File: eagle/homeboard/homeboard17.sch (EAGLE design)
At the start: 128 parts, among them IC1 XCF02S, IC2 25LC080SN, IC3 ATMEGA32U2-TQFP, Q5 BC848SMD, Q6 BC848SMD, Q7 BC848SMD, Q8 BC848SMD, T1 BSS138, T2 BC848, T3 BSS138, T4 BC848, U1 XC3S400TQ144, X1 SCART-CLIP, X6 MINI-USB_4P-85-32004-10X, X7 DC21MMX, X8 STEREOJACK

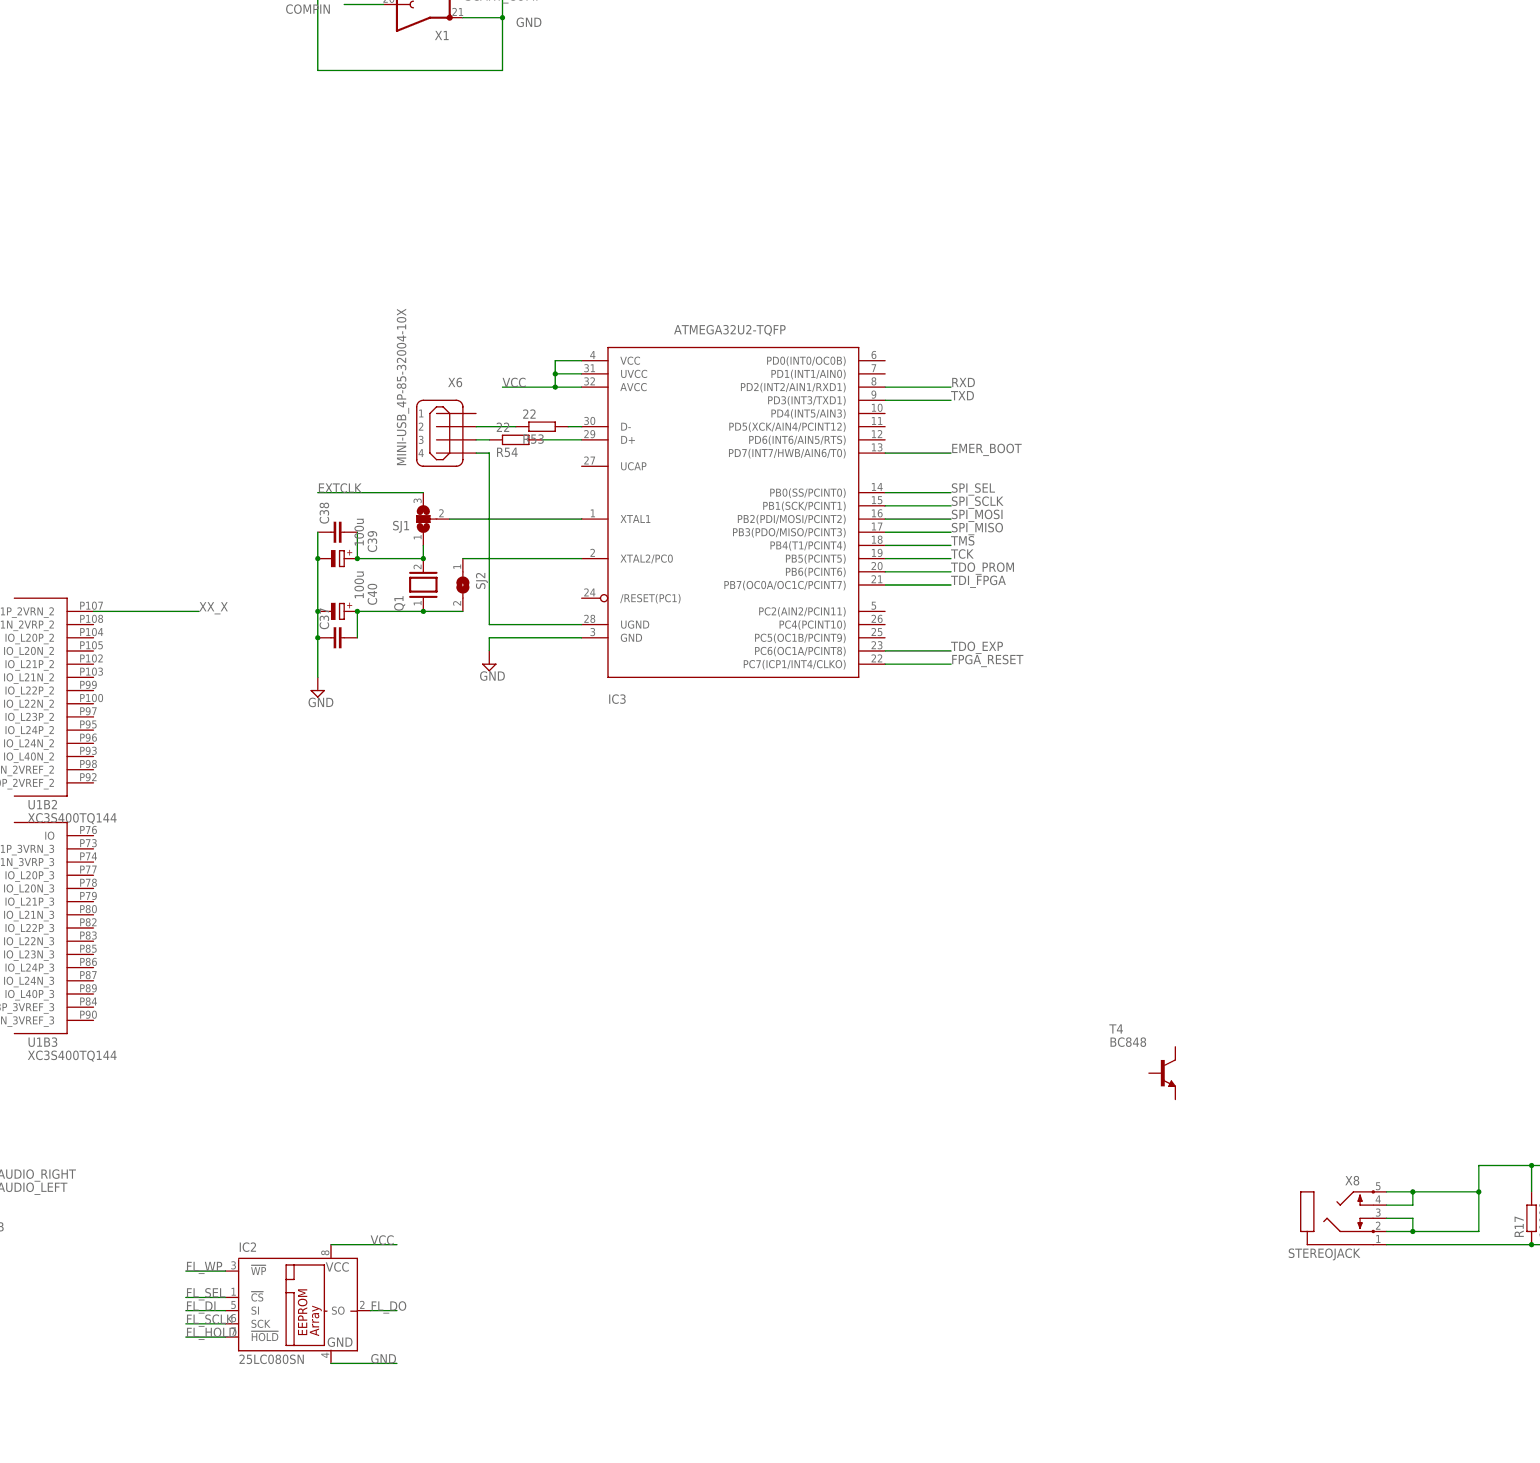
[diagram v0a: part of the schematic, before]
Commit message: mah
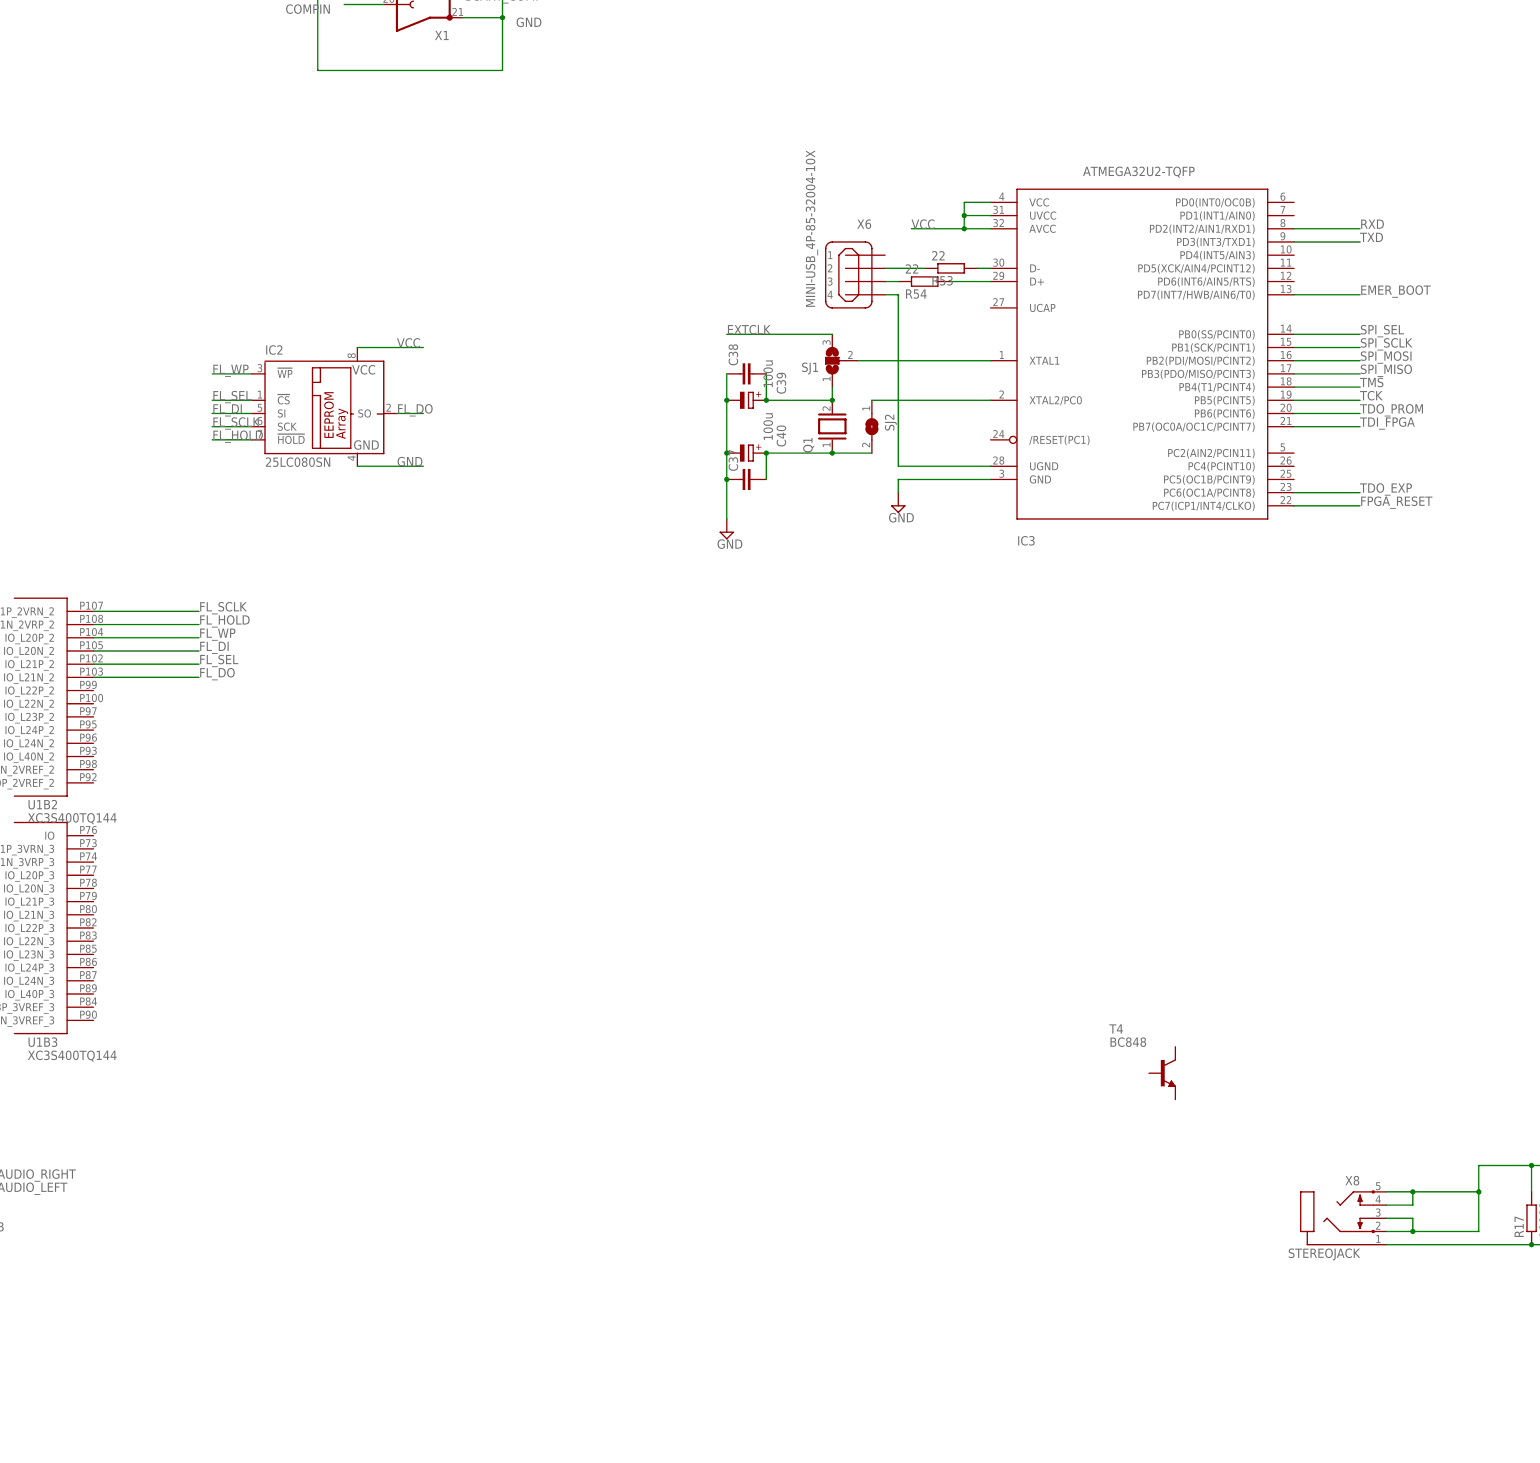
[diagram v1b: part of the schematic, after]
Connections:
- removed net XX_X: U1B2.IO_L01P_2VRN_2
- net FL_DI: now also U1B2.IO_L20N_2
- net FL_DO: now also U1B2.IO_L21N_2
- net FL_HOLD: now also U1B2.IO_L01N_2VRP_2
- net FL_SCLK: now also U1B2.IO_L01P_2VRN_2
- net FL_SEL: now also U1B2.IO_L21P_2
- net FL_WP: now also U1B2.IO_L20P_2
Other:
- moved on the sheet: C37, C38, C39, C40, IC2, IC3, Q1, R53, R54, SJ1, SJ2, X6
